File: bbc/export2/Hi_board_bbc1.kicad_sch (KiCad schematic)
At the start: 15 parts, among them J1 sw-latchboard, J2 led-latchboard, J3 GLVMP, SW1 BSPD_RESET, SW2 IMD_RESET, SW3 BMS_RESET

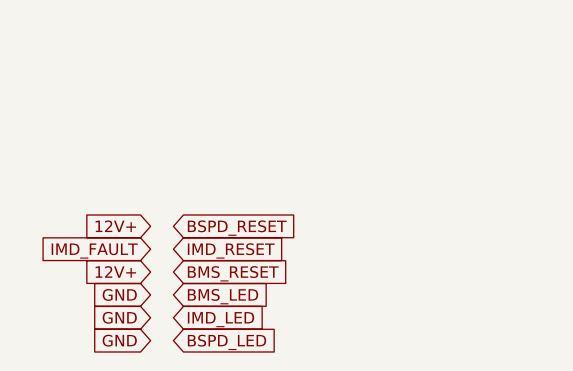
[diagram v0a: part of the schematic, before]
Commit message: Add files via upload
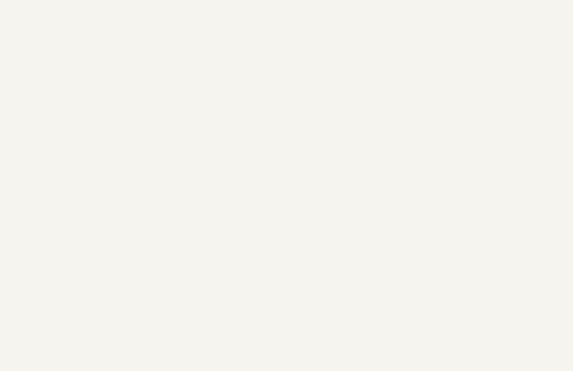
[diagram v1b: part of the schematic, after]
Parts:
- D1, D2, D3: MFG (none) -> Würth Elektronik; MPN (none) -> 151051RS11000
- J3: footprint (none) -> GLVMP_Banana_Jack:GLVMP_Banana_Jack
- R1, R2, R3, R4, R5, R6: MFG (none) -> Stackpole Electronics Inc; MPN (none) -> CF14JT220R
- SW1, SW2, SW3: MFG (none) -> TE Connectivity ALCOSWITCH Switches; MPN (none) -> 2-1825910-7

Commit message: Add files via upload
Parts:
- J1, J2: MFG (none) -> Molex; MPN (none) -> 39281063
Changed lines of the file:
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@@
 			)
 		)
-		(property "MFG" ""
+		(property "MFG" "Molex"
 			(at 146.05 86.36 0)
 			(effects
@@
 			)
 		)
-		(property "MPN" ""
+		(property "MPN" "39281063"
 			(at 146.05 86.36 0)
 			(effects
@@
 			)
 		)
-		(property "MFG" ""
+		(property "MFG" "Molex"
 			(at 144.78 64.77 0)
 			(effects
@@
 			)
 		)
-		(property "MPN" ""
+		(property "MPN" "39281063"
 			(at 144.78 64.77 0)
 			(effects
